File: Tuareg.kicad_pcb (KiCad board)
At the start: 4 copper layers, 101.6 x 103.6 mm, 202 parts, among them CON1 ModICE_48, J1 SWD_boctok, P1 VNLD5090e, P2 FAN1100, P3 VNLD5090e, P4 FAN1100, P5 ISO7421D, Q1 BTS3028SDL, Q2 BTS3028SDL, Q3 ISL9V3040, Q4 BTS3028SDL, Q5 ISL9V3040, U1 NCV1117DT, U2 NCV1117ST, U3 MCP6004, U4 MCP6004, U5 LM2903, U6 STM32F410RBTx, U7 24C64, Y1 lfxtal071673, Y2 cx5032ga

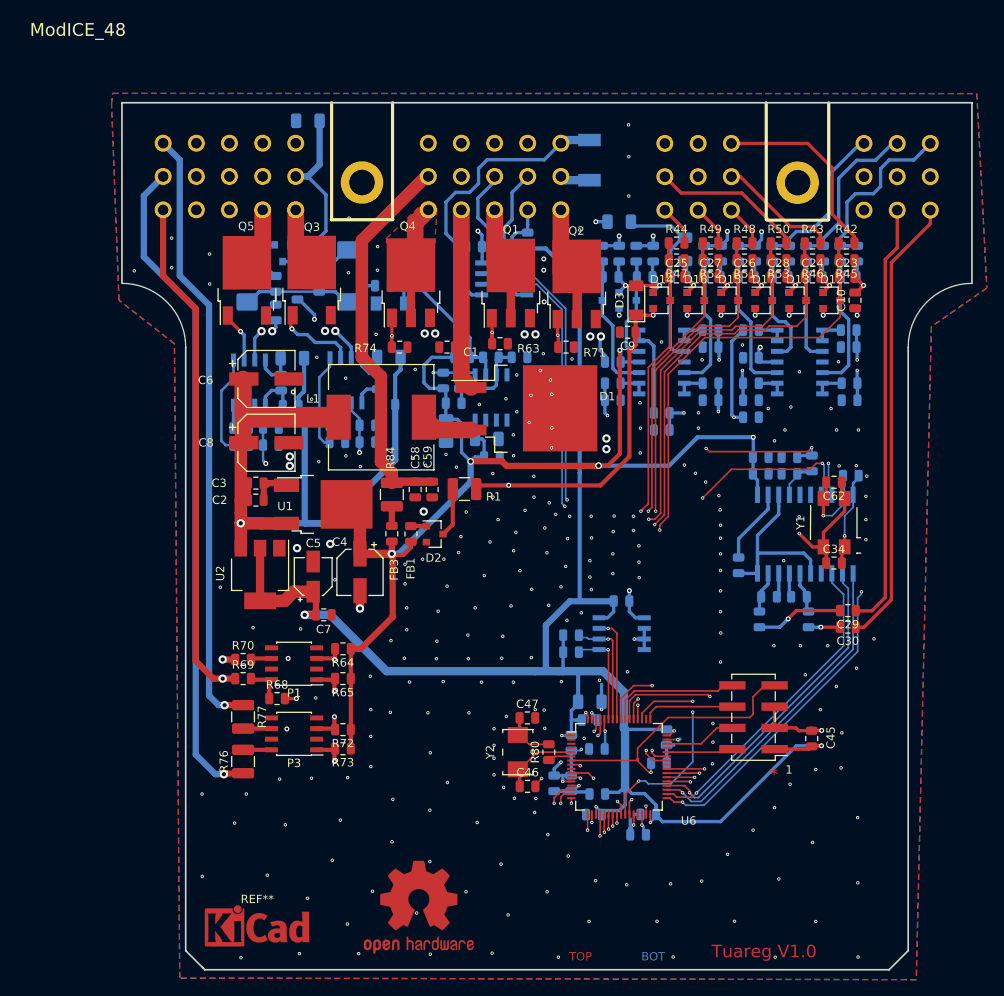
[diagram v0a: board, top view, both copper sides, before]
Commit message: cleaning up
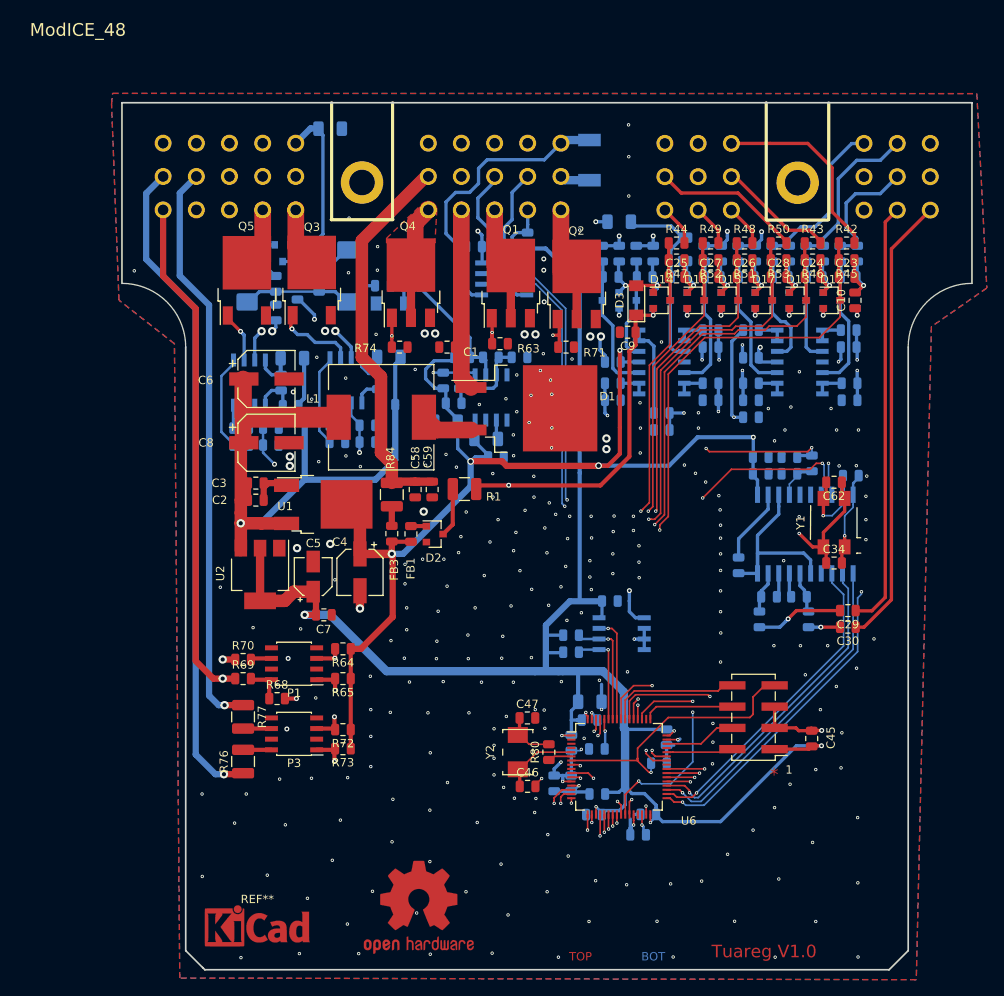
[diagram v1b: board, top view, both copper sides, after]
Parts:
- moved R34 2.82 mm to (102.6, 54.9), turned to 0 degrees
- moved C44 1.39 mm to (136.0, 111.4)
- moved C64 1.12 mm to (116.5, 89.9), turned to 180 degrees
- moved C63 0.48 mm to (122.4, 94.2)
- moved C22 0.08 mm to (121.3, 92.0)
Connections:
- CON1 pad 13: /con_ach4 -> GND
- CON1 pad 34: /con_vrcrank+ -> GND
- CON1 pad 37: GND -> /con_spareact2
- CON1 pad 44: GND -> /con_vrcrank+
- CON1 pad 48: /con_spareact2 -> GND
- CON1 pad 8: GND -> /con_ach4
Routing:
- net GND: track 467.0 -> 477.4 mm, vias 282 -> 278
- net /con_ach8: track 41.1 -> 33.3 mm
- net +12V: track 203.7 -> 196.5 mm
- net /con_ach4: track 21.7 -> 15.1 mm
- net /con_spareact2: track 72.8 -> 68.8 mm
- net +5V: track 183.6 -> 180.8 mm
- net +3V3: track 212.4 -> 209.8 mm
- net /INJ2: track 72.7 -> 74.2 mm
- net /con_ach2: track 19.2 -> 19.8 mm
- net Net-(P4-Pad5): track 11.9 -> 11.4 mm
